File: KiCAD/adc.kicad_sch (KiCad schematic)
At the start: 4 parts, among them IC1 ADS7953SBDBTR, IC2 ADS7953SBDBTR, IC3 ADS7953SBDBTR, IC4 ADS7953SBDBTR

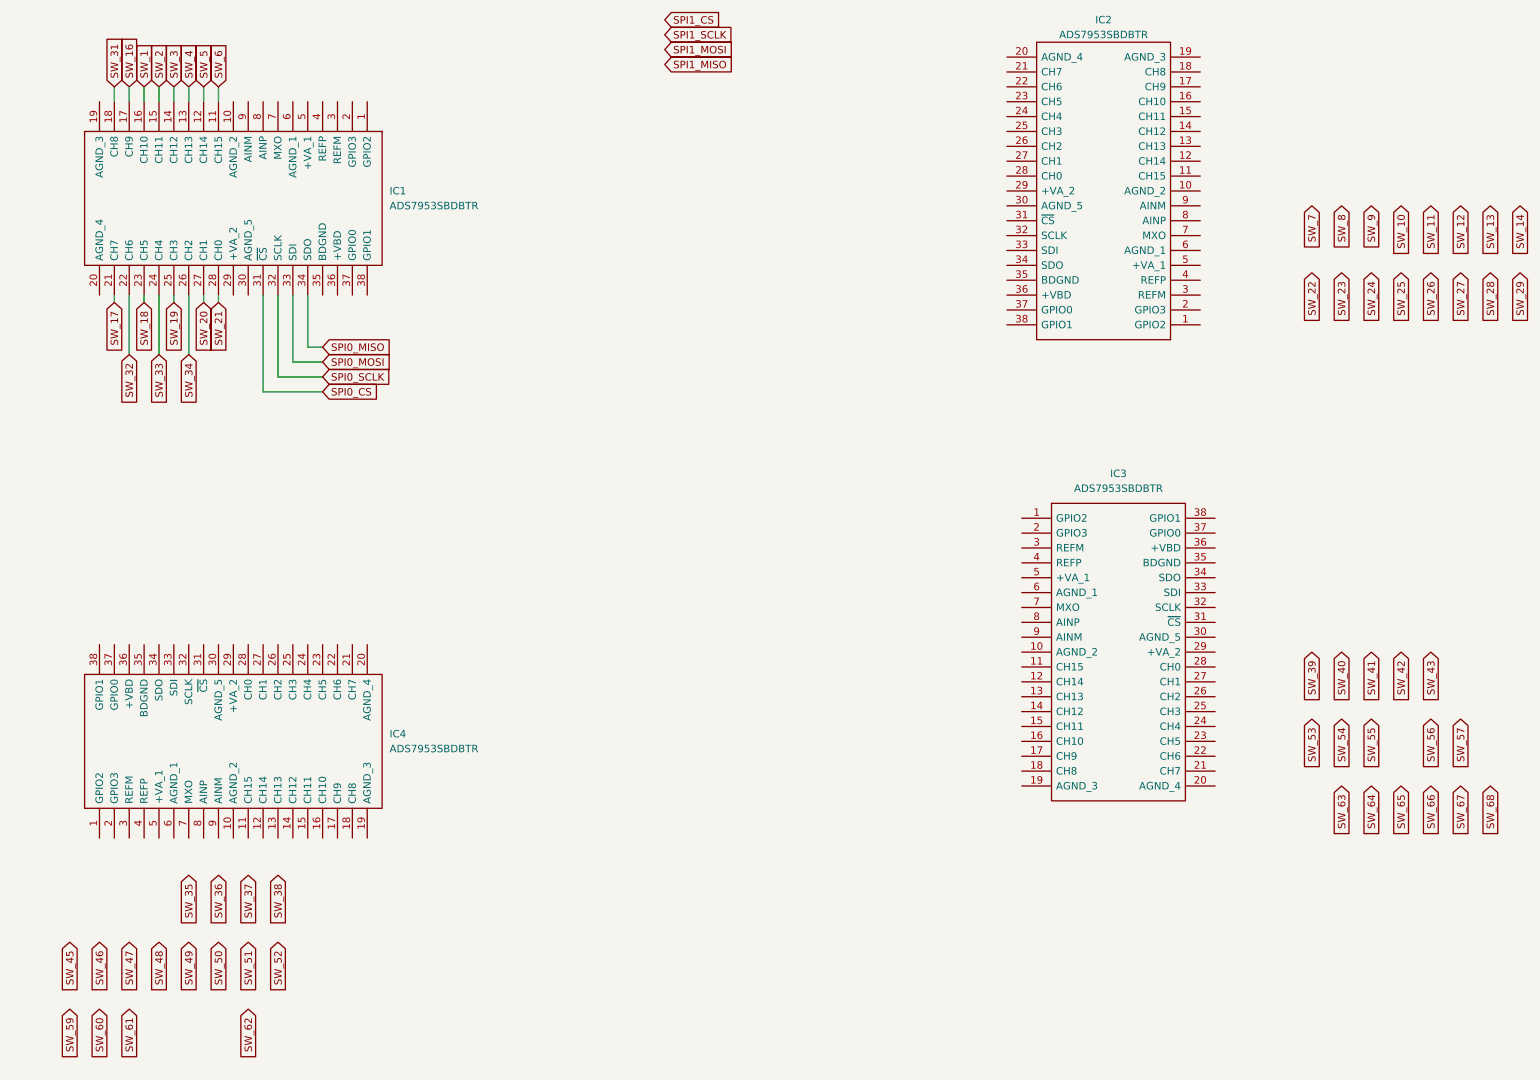
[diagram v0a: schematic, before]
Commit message: Committing before changing to MUX design
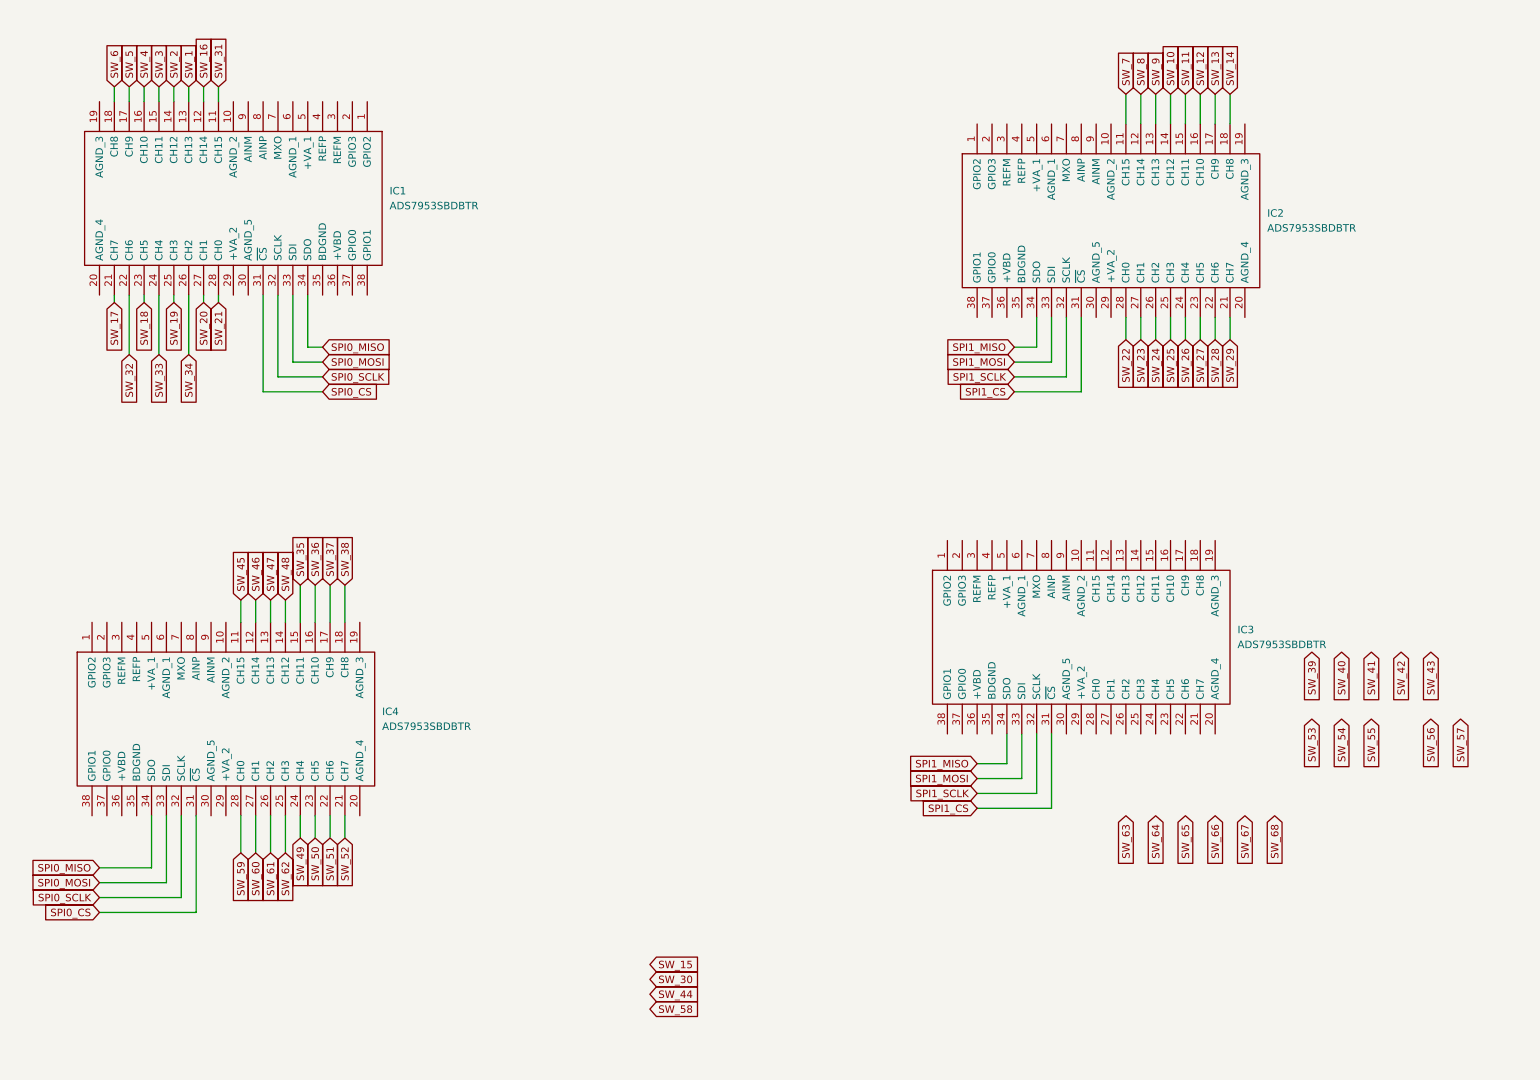
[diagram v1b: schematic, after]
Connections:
- net SPI0_CS: now also IC4.31 (~{CS})
- net SPI0_MISO: now also IC4.34 (SDO)
- net SPI0_MOSI: now also IC4.33 (SDI)
- net SPI0_SCLK: now also IC4.32 (SCLK)
- net SPI1_CS: now also IC2.31 (~{CS}), IC3.31 (~{CS})
- net SPI1_MISO: now also IC2.34 (SDO), IC3.34 (SDO)
- net SPI1_MOSI: now also IC2.33 (SDI), IC3.33 (SDI)
- net SPI1_SCLK: now also IC2.32 (SCLK), IC3.32 (SCLK)
- net SW_1: now also IC1.13 (CH13); no longer IC1.16 (CH10)
- net SW_10: now also IC2.14 (CH12)
- net SW_11: now also IC2.15 (CH11)
- net SW_12: now also IC2.16 (CH10)
- net SW_13: now also IC2.17 (CH9)
- net SW_14: now also IC2.18 (CH8)
- net SW_16: now also IC1.12 (CH14); no longer IC1.17 (CH9)
- net SW_2: now also IC1.14 (CH12); no longer IC1.15 (CH11)
- net SW_22: now also IC2.28 (CH0)
- net SW_23: now also IC2.27 (CH1)
- net SW_24: now also IC2.26 (CH2)
- net SW_25: now also IC2.25 (CH3)
- net SW_26: now also IC2.24 (CH4)
- net SW_27: now also IC2.23 (CH5)
- net SW_28: now also IC2.22 (CH6)
- net SW_29: now also IC2.21 (CH7)
- net SW_3: now also IC1.15 (CH11); no longer IC1.14 (CH12)
- net SW_31: now also IC1.11 (CH15); no longer IC1.18 (CH8)
- net SW_35: now also IC4.15 (CH11)
- net SW_36: now also IC4.16 (CH10)
- net SW_37: now also IC4.17 (CH9)
- net SW_38: now also IC4.18 (CH8)
- net SW_4: now also IC1.16 (CH10); no longer IC1.13 (CH13)
- net SW_45: now also IC4.11 (CH15)
- net SW_46: now also IC4.12 (CH14)
- net SW_47: now also IC4.13 (CH13)
- net SW_48: now also IC4.14 (CH12)
- net SW_49: now also IC4.24 (CH4)
- net SW_5: now also IC1.17 (CH9); no longer IC1.12 (CH14)
- net SW_50: now also IC4.23 (CH5)
- net SW_51: now also IC4.22 (CH6)
- net SW_52: now also IC4.21 (CH7)
- net SW_59: now also IC4.28 (CH0)
- net SW_6: now also IC1.18 (CH8); no longer IC1.11 (CH15)
- net SW_60: now also IC4.27 (CH1)
- net SW_61: now also IC4.26 (CH2)
- net SW_62: now also IC4.25 (CH3)
- net SW_7: now also IC2.11 (CH15)
- net SW_8: now also IC2.12 (CH14)
- net SW_9: now also IC2.13 (CH13)
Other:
- moved on the sheet: IC2, IC3, IC4

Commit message: Finished initial routing of PCB
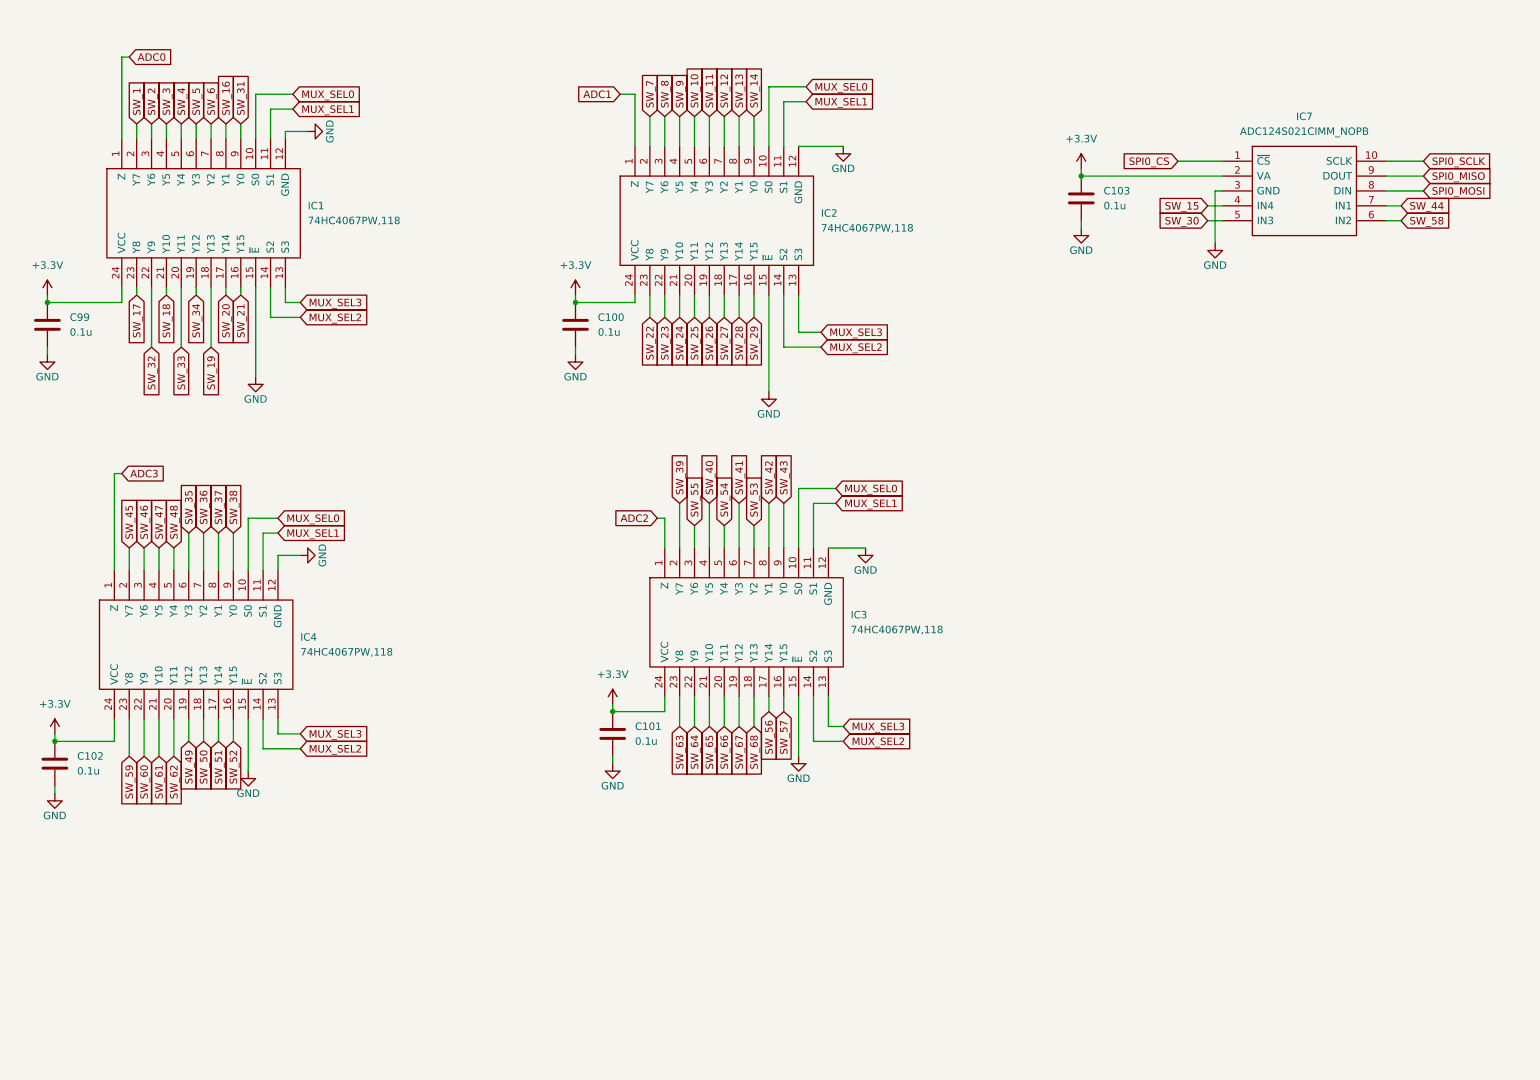
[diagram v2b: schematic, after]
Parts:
- removed IC1, IC2, IC3, IC4: ADS7953SBDBTR, Package_SO:TSSOP-38_4.4x9.7mm_P0.5mm, symbol SamacSys_Parts:ADS7953SBDBTR
- added C100, C101, C102, C103, C99: 0.1u, Capacitor_SMD:C_0603_1608Metric_Pad1.08x0.95mm_HandSolder, symbol Device:C
- added IC1, IC2, IC3, IC4: 74HC4067PW,118, SamacSys_Parts:SOP65P640X110-24N, symbol SamacSys_Parts:74HC4067PW,118
- added IC7: ADC124S021CIMM_NOPB, SamacSys_Parts:SOP50P490X110-10N, symbol SamacSys_Parts:ADC124S021CIMM_NOPB
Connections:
- net SPI0_CS: now also IC7.1 (~{CS})
- net SPI0_MISO: now also IC7.9 (DOUT)
- net SPI0_MOSI: now also IC7.8 (DIN)
- net SPI0_SCLK: now also IC7.10 (SCLK)
- net SW_1: now also IC1.2 (Y7)
- net SW_10: now also IC2.5 (Y4)
- net SW_11: now also IC2.6 (Y3)
- net SW_12: now also IC2.7 (Y2)
- net SW_13: now also IC2.8 (Y1)
- net SW_14: now also IC2.9 (Y0)
- net SW_15: now also IC7.4 (IN4)
- net SW_16: now also IC1.8 (Y1)
- net SW_17: now also IC1.23 (Y8)
- net SW_18: now also IC1.21 (Y10)
- net SW_19: now also IC1.18 (Y13)
- net SW_2: now also IC1.3 (Y6)
- net SW_20: now also IC1.17 (Y14)
- net SW_21: now also IC1.16 (Y15)
- net SW_22: now also IC2.23 (Y8)
- net SW_23: now also IC2.22 (Y9)
- net SW_24: now also IC2.21 (Y10)
- net SW_25: now also IC2.20 (Y11)
- net SW_26: now also IC2.19 (Y12)
- net SW_27: now also IC2.18 (Y13)
- net SW_28: now also IC2.17 (Y14)
- net SW_29: now also IC2.16 (Y15)
- net SW_3: now also IC1.4 (Y5)
- net SW_30: now also IC7.5 (IN3)
- net SW_31: now also IC1.9 (Y0)
- net SW_32: now also IC1.22 (Y9)
- net SW_33: now also IC1.20 (Y11)
- net SW_34: now also IC1.19 (Y12)
- net SW_35: now also IC4.6 (Y3)
- net SW_36: now also IC4.7 (Y2)
- net SW_37: now also IC4.8 (Y1)
- net SW_38: now also IC4.9 (Y0)
- net SW_39: now also IC3.2 (Y7)
- net SW_4: now also IC1.5 (Y4)
- net SW_40: now also IC3.4 (Y5)
- net SW_41: now also IC3.6 (Y3)
- net SW_42: now also IC3.8 (Y1)
- net SW_43: now also IC3.9 (Y0)
- net SW_44: now also IC7.7 (IN1)
- net SW_45: now also IC4.2 (Y7)
- net SW_46: now also IC4.3 (Y6)
- net SW_47: now also IC4.4 (Y5)
- net SW_48: now also IC4.5 (Y4)
- net SW_49: now also IC4.19 (Y12)
- net SW_5: now also IC1.6 (Y3)
- net SW_50: now also IC4.18 (Y13)
- net SW_51: now also IC4.17 (Y14)
- net SW_52: now also IC4.16 (Y15)
- net SW_53: now also IC3.7 (Y2)
- net SW_54: now also IC3.5 (Y4)
- net SW_55: now also IC3.3 (Y6)
- net SW_56: now also IC3.17 (Y14)
- net SW_57: now also IC3.16 (Y15)
- net SW_58: now also IC7.6 (IN2)
- net SW_59: now also IC4.23 (Y8)
- net SW_6: now also IC1.7 (Y2)
- net SW_60: now also IC4.22 (Y9)
- net SW_61: now also IC4.21 (Y10)
- net SW_62: now also IC4.20 (Y11)
- net SW_63: now also IC3.23 (Y8)
- net SW_64: now also IC3.22 (Y9)
- net SW_65: now also IC3.21 (Y10)
- net SW_66: now also IC3.20 (Y11)
- net SW_67: now also IC3.19 (Y12)
- net SW_68: now also IC3.18 (Y13)
- net SW_7: now also IC2.2 (Y7)
- net SW_8: now also IC2.3 (Y6)
- net SW_9: now also IC2.4 (Y5)
- new net +3V3: C100.1, C101.1, C102.1, C103.1, C99.1, IC1.24 (VCC), IC2.24 (VCC), IC3.24 (VCC), IC4.24 (VCC), IC7.2 (VA)
- new net ADC0: IC1.1 (Z)
- new net ADC1: IC2.1 (Z)
- new net ADC2: IC3.1 (Z)
- new net ADC3: IC4.1 (Z)
- new net GND: C100.2, C101.2, C102.2, C103.2, C99.2, IC1.12 (GND), IC1.15 (~{E}), IC2.12 (GND), IC2.15 (~{E}), IC3.12 (GND), IC3.15 (~{E}), IC4.12 (GND), IC4.15 (~{E}), IC7.3 (GND)
- new net MUX_SEL0: IC1.10 (S0), IC2.10 (S0), IC3.10 (S0), IC4.10 (S0)
- new net MUX_SEL1: IC1.11 (S1), IC2.11 (S1), IC3.11 (S1), IC4.11 (S1)
- new net MUX_SEL2: IC1.14 (S2), IC2.14 (S2), IC3.14 (S2), IC4.14 (S2)
- new net MUX_SEL3: IC1.13 (S3), IC2.13 (S3), IC3.13 (S3), IC4.13 (S3)
